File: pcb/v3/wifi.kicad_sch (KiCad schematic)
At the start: 17 parts, among them U11 TXS0102DCU, U12 TXS0102DCU, U8 M8800DU6, U9 SY6280

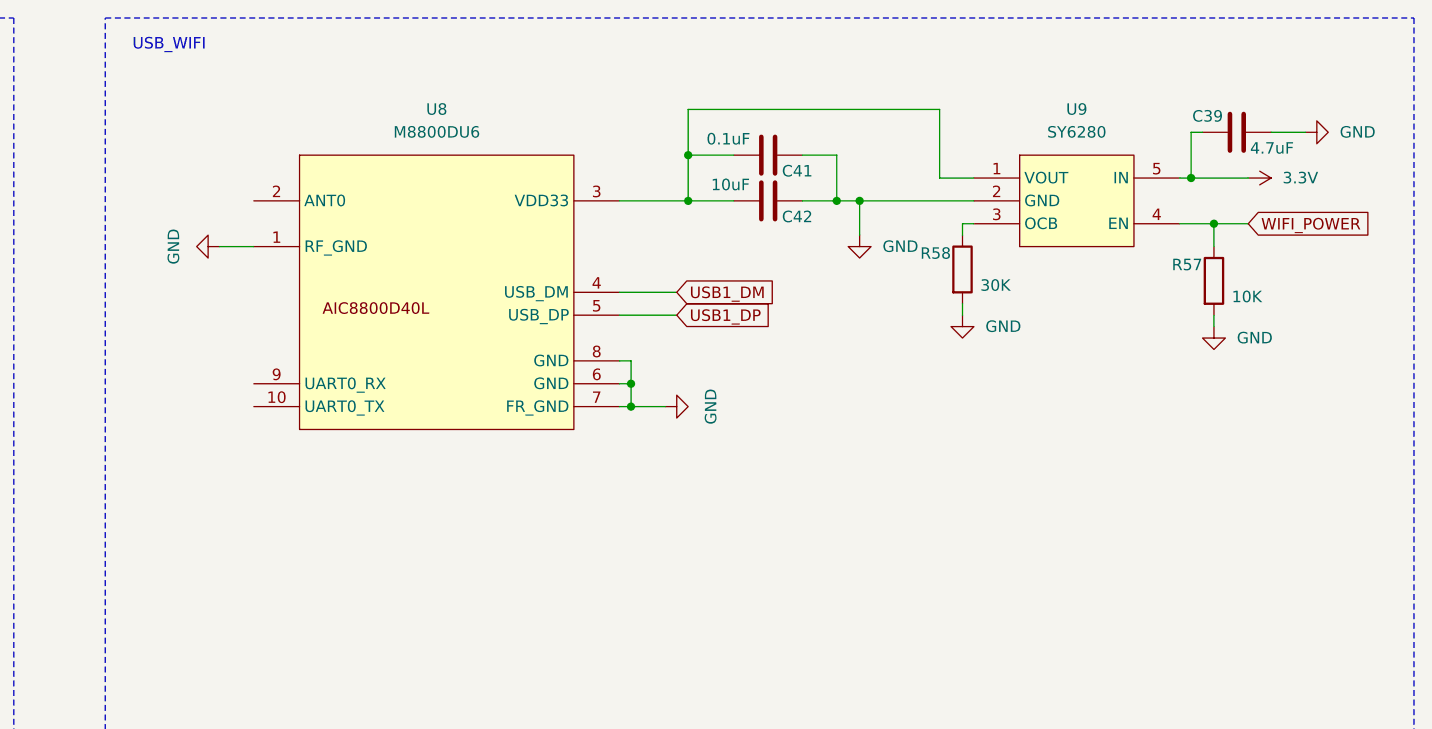
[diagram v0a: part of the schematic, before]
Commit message: up
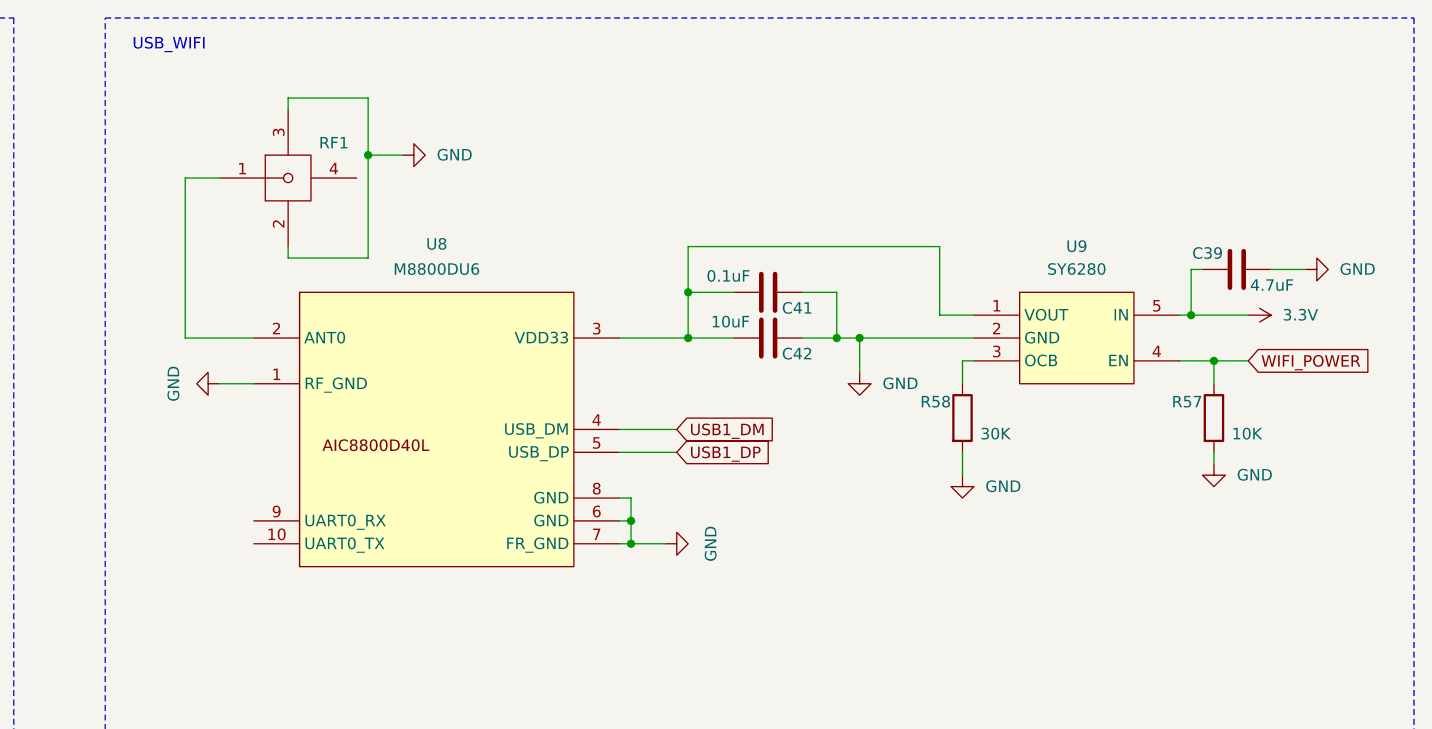
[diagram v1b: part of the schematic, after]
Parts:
- added RF1: 6GHz, coloryr:IPEX-SMD_BWIPX-3-001E-1, symbol coloryr:BWIPX-3-001E
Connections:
- net GND: now also RF1.2, RF1.3
- net at U8.2 (ANT0): now also RF1.1
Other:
- moved on the sheet: C39, C41, C42, R57, R58, U8, U9

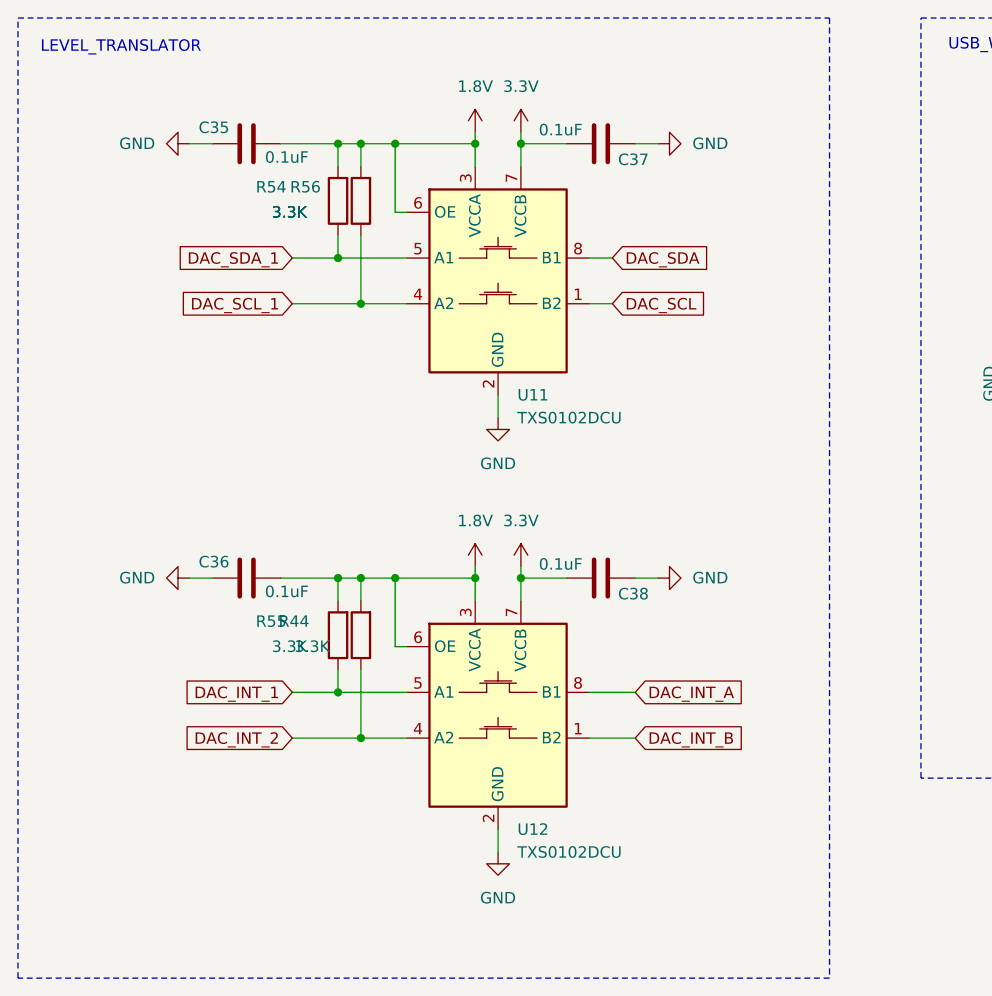
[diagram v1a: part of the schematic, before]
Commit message: up
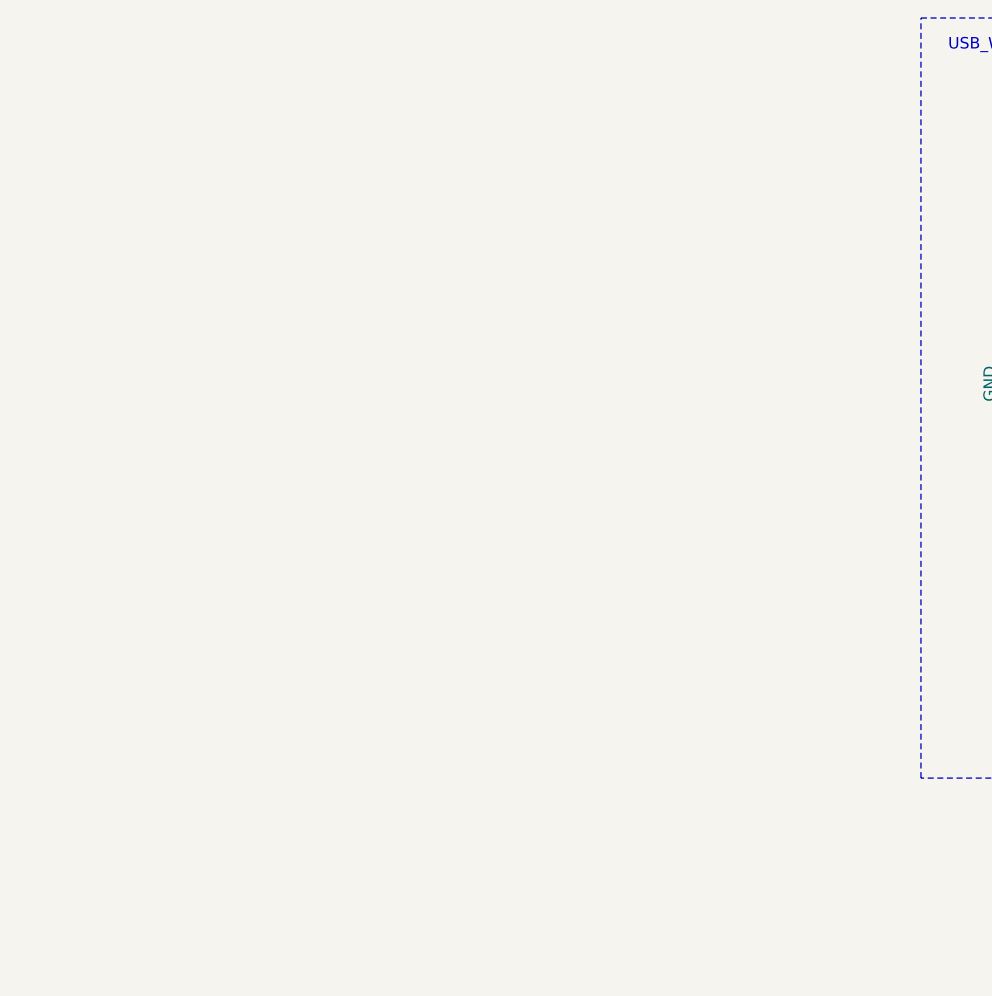
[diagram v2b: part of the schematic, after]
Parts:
- removed C35, C36, C37, C38: 0.1uF, Capacitor_SMD:C_0402_1005Metric_Pad0.74x0.62mm_HandSolder, symbol Device:C
- removed R44, R54, R55, R56: 3.3K, Capacitor_SMD:C_0402_1005Metric_Pad0.74x0.62mm_HandSolder, symbol Device:R
- removed U11, U12: TXS0102DCU, Package_SO:VSSOP-8_2.3x2mm_P0.5mm, symbol Logic_LevelTranslator:TXS0102DCU
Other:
- note removed: "LEVEL_TRANSLATOR"

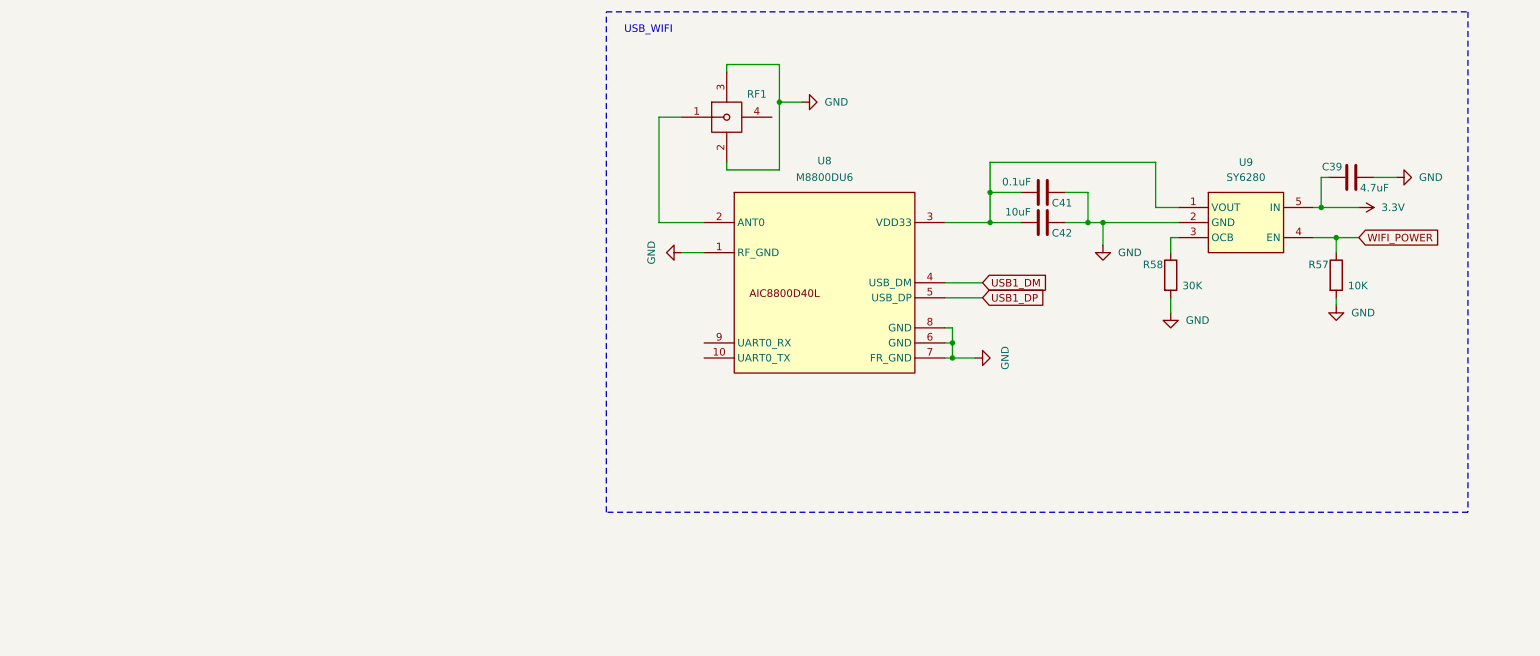
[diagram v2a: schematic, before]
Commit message: pcb 3.9
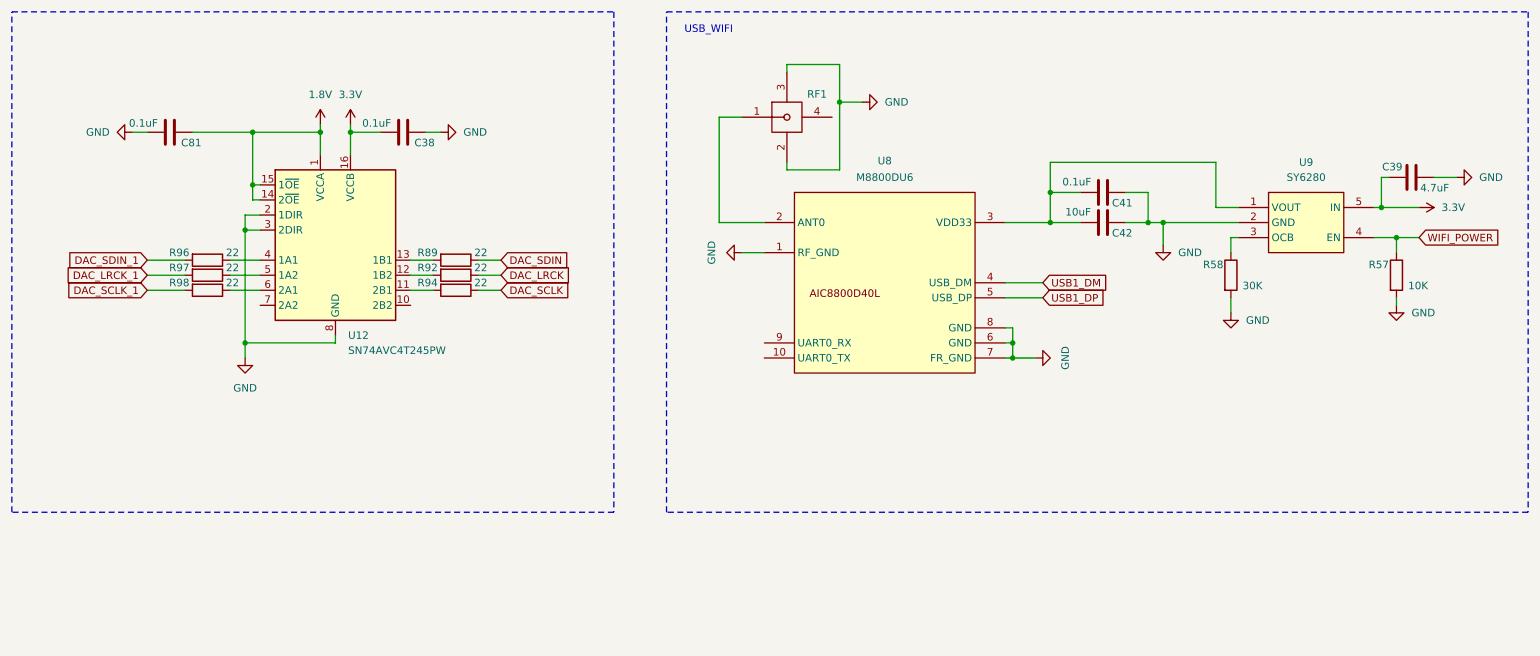
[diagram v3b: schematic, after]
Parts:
- added C38, C81: 0.1uF, Capacitor_SMD:C_0402_1005Metric_Pad0.74x0.62mm_HandSolder, symbol Device:C
- added R89, R92, R94, R96, R97, R98: 22, Capacitor_SMD:C_0402_1005Metric_Pad0.74x0.62mm_HandSolder, symbol Device:R
- added U12: SN74AVC4T245PW, Package_DFN_QFN:UQFN-16_1.8x2.6mm_P0.4mm, symbol Logic_LevelTranslator:SN74AVC4T245PW
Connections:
- net 3.3V: now also C38.1, U12.16 (VCCB)
- net GND: now also C38.2, C81.1, U12.2 (1DIR), U12.3 (2DIR), U12.8 (GND), U12.9 (GND)
- new net: R92.2, U12.12 (1B2)
- new net: R94.2, U12.11 (2B1)
- new net: R89.2, U12.13 (1B1)
- new net: R96.1, U12.4 (1A1)
- new net: R97.1, U12.5 (1A2)
- new net: R98.1, U12.6 (2A1)
- new net 1.8V: C81.2, U12.1 (VCCA), U12.14 (2~{OE}), U12.15 (1~{OE})
- new net DAC_LRCK: R92.1
- new net DAC_LRCK_1: R97.2
- new net DAC_SCLK: R94.1
- new net DAC_SCLK_1: R98.2
- new net DAC_SDIN: R89.1
- new net DAC_SDIN_1: R96.2
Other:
- moved on the sheet: C39, C41, C42, R57, R58, RF1, U8, U9
